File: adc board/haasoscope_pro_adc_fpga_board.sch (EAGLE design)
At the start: 563 parts, among them CN2 12Vin, IC1 ADC12DL2500ACF, IC13 LMH5401IRMST, IC14 LMH6401IRMZR, IC15 SN74AVC4T774PWR, IC17 DAC8562SDGSR, IC18 TLV9102IPWR, IC2 SN74AVC4T774PWR, IC21 LMH5401IRMST, IC22 TPS7A7200RGTR, IC23 TPS7A7200RGTR, IC24 TPS7A7200RGTR, IC25 TPS72325DBVR, IC26 TPS7A7200RGTR, IC27 TPS7A7200RGTR, IC28 TPS7A7200RGTR, IC29 LMH6401IRMZR, IC3 ADC122S021CIMM_NOPB, IC30 SN74AVC4T774PWR, IC33 TLV9102IPWR, IC4 TLV9102IPWR, IC5 EP4CE30F23C6N, IC6 EPCQ16ASI8N, IC8 FT232HQ, IC9 93LC56B, J1 2p-2.54, J10 8pin, J11 8pin, J13 8pin, J14 2x5, J15 test1, J2 test1, J30 2p-2.54, J31 2p-2.54, J32 2p-2.54, J33 2p-2.54, J34 2p-2.54, J35 2p-2.54, J36 2p-2.54, J37 2p-2.54, J39 2p-2.54, J40 2p-2.54, J41 2p-2.54, J42 2p-2.54, J43 2p-2.54, J44 2p-2.54, J45 2p-2.54, J46 2p-2.54, J8 8pin, K10 G6K-2F-RF-DC3, K11 G6K-2F-RF-DC3, K12 G6K-2F-RF-DC3, K5 AQY21SOP, K6 G6K-2F-RF-DC3, K7 G6K-2F-RF-DC3, K9 AQY21SOP, Q1 S8050, Q4 S8050, Q5 S8050, Q7 S8050, Q8 S8050, Q9 S8050, SW3 SKQGADE010, SW4 SKQGADE010, U2 ADF4350BCPZ, U6 AMS1117-1.2, X1 USBC, Y2 OSCILLATORSMD-5X3, Y3 12MHz

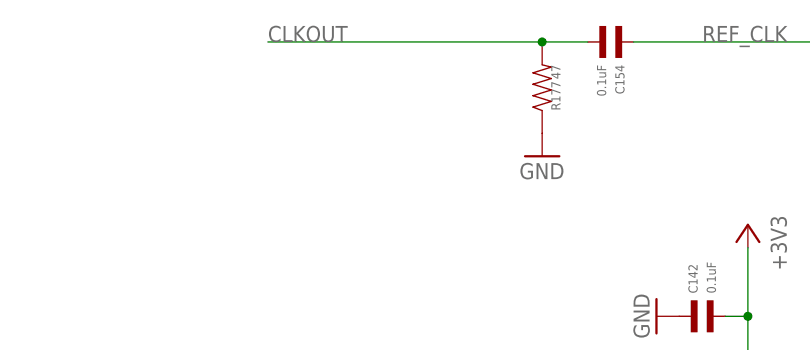
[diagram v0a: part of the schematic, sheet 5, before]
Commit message: put back clk cap
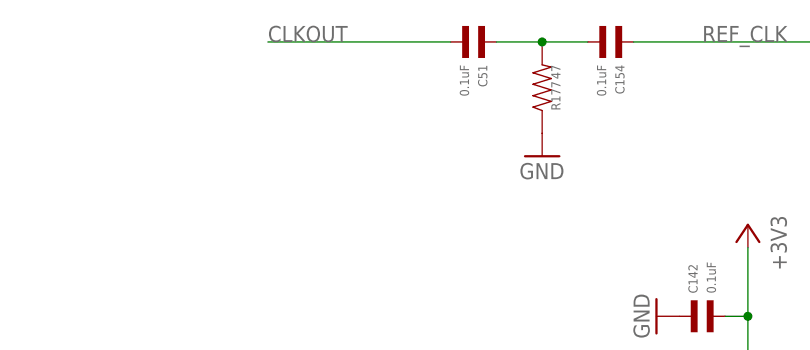
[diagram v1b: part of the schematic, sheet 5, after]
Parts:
- added C51: 0.1uF, MF_Passives:CAPACITOR_NP_0402
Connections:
- new net N$11: C154.P$2, C51.P$1, R177.P$2
- net CLKOUT: now also C51.P$2; no longer C154.P$2, R177.P$2
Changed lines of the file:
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@@
 <part name="R208" library="MF_Passives" deviceset="RESISTOR" device="_0402" value="1k"/>
 <part name="JST_FAN" library="SparkFun-Connectors" deviceset="M02" device="PTH" value="Fan"/>
+<part name="C51" library="MF_Passives" deviceset="CAPACITOR_NP" device="_0402" value="0.1uF"/>
 </parts>
 <sheets>
@@
 <attribute name="VALUE" x="111.76" y="78.74" size="1.778" layer="96"/>
 </instance>
+<instance part="C51" gate="G$1" x="160.02" y="226.06" smashed="yes" rot="R270">
+<attribute name="NAME" x="161.544" y="223.52" size="1.016" layer="95" font="vector" rot="R270" align="top-left"/>
+<attribute name="VALUE" x="158.496" y="223.52" size="1.016" layer="96" font="vector" rot="R270"/>
+</instance>
 </instances>
 <busses>
@@
 <net name="CLKOUT" class="5">
 <segment>
-<wire x1="137.16" y1="226.06" x2="167.64" y2="226.06" width="0.1524" layer="91"/>
 <label x="137.16" y="226.06" size="1.778" layer="95"/>
-<pinref part="R177" gate="G$1" pin="P$2"/>
-<pinref part="C154" gate="G$1" pin="P$2"/>
-<wire x1="167.64" y1="226.06" x2="172.72" y2="226.06" width="0.1524" layer="91"/>
-<junction x="167.64" y="226.06"/>
+<wire x1="137.16" y1="226.06" x2="157.48" y2="226.06" width="0.1524" layer="91"/>
+<pinref part="C51" gate="G$1" pin="P$2"/>
 </segment>
 </net>
@@
 </segment>
 </net>
+<net name="N$11" class="5">
+<segment>
+<pinref part="C154" gate="G$1" pin="P$2"/>
+<pinref part="R177" gate="G$1" pin="P$2"/>
+<wire x1="167.64" y1="226.06" x2="172.72" y2="226.06" width="0.1524" layer="91"/>
+<junction x="167.64" y="226.06"/>
+<wire x1="162.56" y1="226.06" x2="167.64" y2="226.06" width="0.1524" layer="91"/>
+<pinref part="C51" gate="G$1" pin="P$1"/>
+</segment>
+</net>
